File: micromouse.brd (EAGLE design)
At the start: 100 x 80 mm, 25 parts

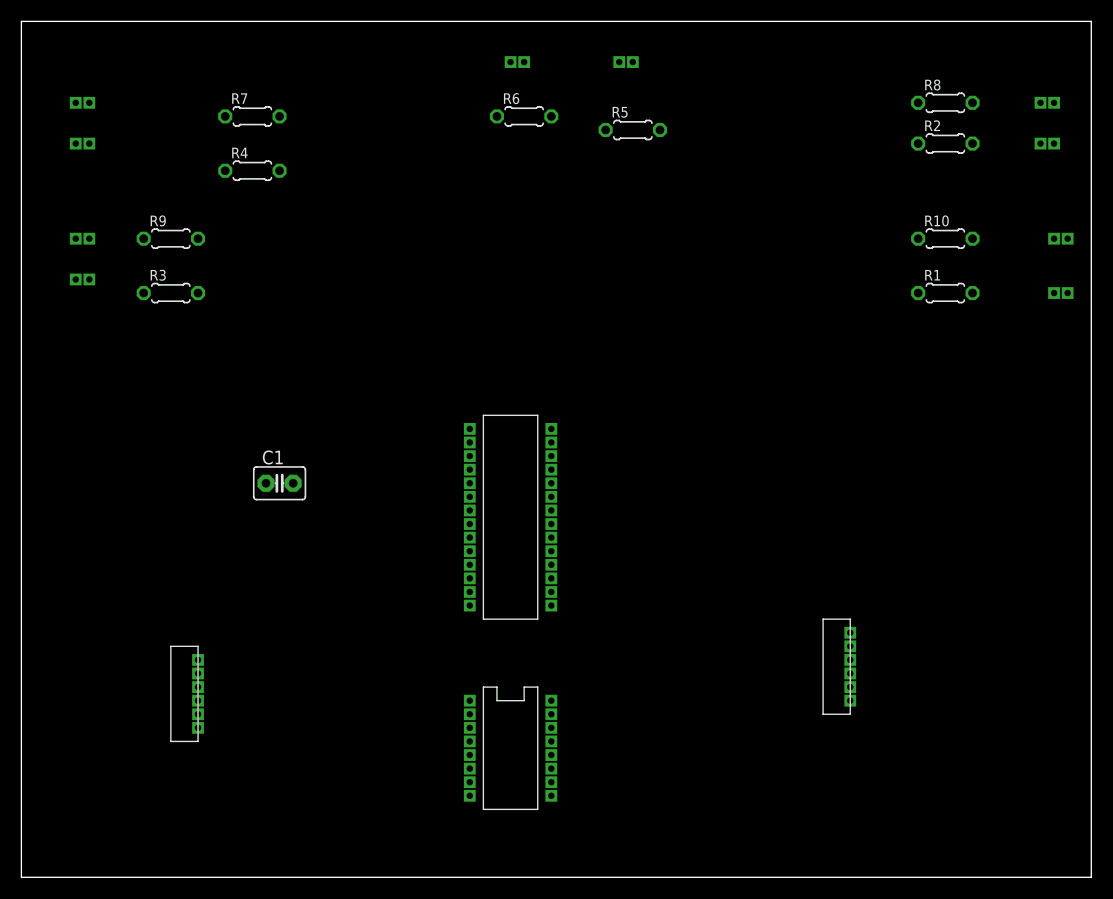
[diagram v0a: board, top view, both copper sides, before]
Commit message: Add files via upload
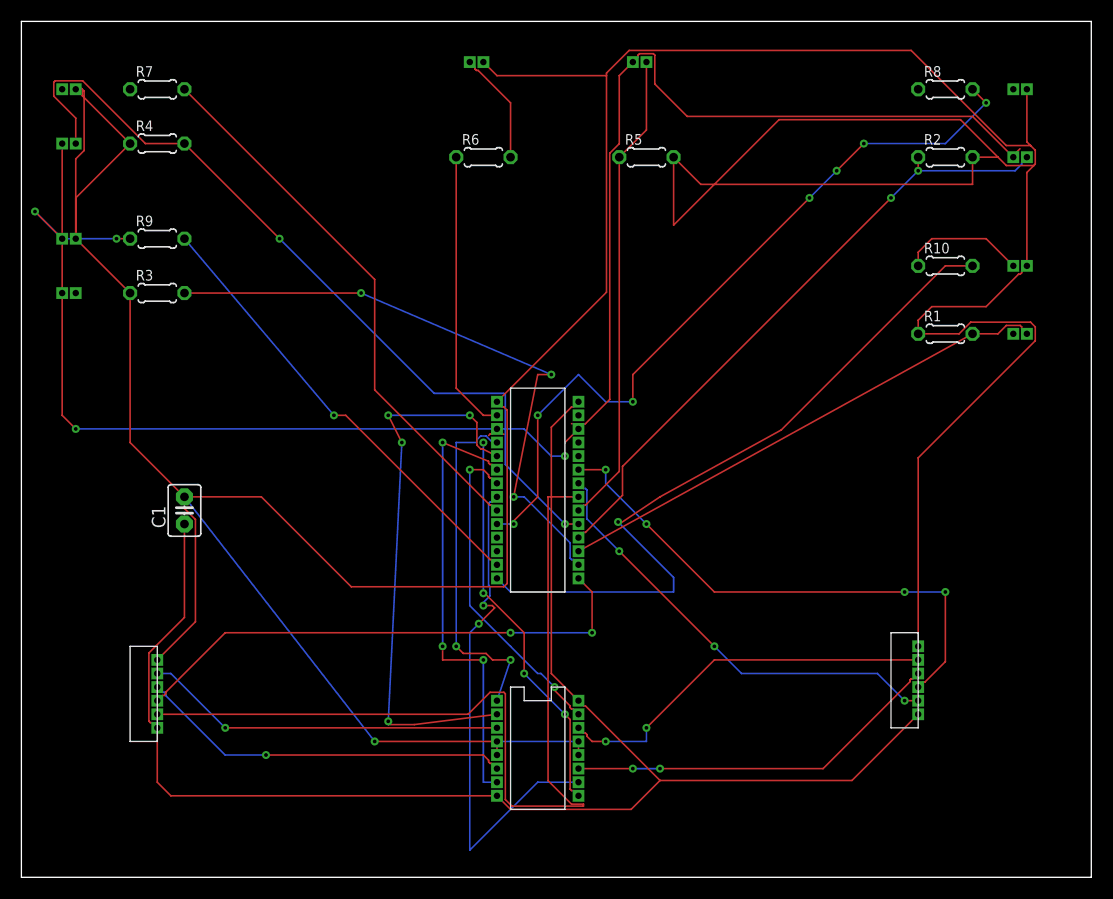
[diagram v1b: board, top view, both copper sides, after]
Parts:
- moved C1 9.25 mm to (15.2, 34.3), turned to 90 degrees
- moved R4 9.25 mm to (12.7, 68.6)
- moved R7 9.25 mm to (12.7, 73.7)
- moved U$14 6.48 mm to (85.1, 19.1)
- moved R6 5.39 mm to (43.2, 67.3)
- moved U$4 5.39 mm to (94.0, 50.8)
- moved U$12 4.58 mm to (94.0, 57.1)
- moved R1 3.81 mm to (86.4, 50.8)
- moved U$8 3.81 mm to (43.2, 76.2)
- moved U$13 3.81 mm to (14.0, 17.8)
- moved U$1 3.59 mm to (48.3, 36.8)
- moved R5 2.84 mm to (58.4, 67.3)
- moved U$10 2.84 mm to (94.0, 73.7)
- moved U$5 2.84 mm to (94.0, 67.3)
- moved R10 2.54 mm to (86.4, 57.1)
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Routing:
- net GND: track 0.00 -> 428.1 mm, vias 0 -> 1
- net N$36: track 0.00 -> 156.3 mm, vias 0 -> 2
- net N$30: track 0.00 -> 142.6 mm
- net N$29: track 0.00 -> 84.7 mm
- net N$21: track 0.00 -> 77.5 mm, vias 0 -> 2
- net N$14: track 0.00 -> 72.5 mm, vias 0 -> 7
- net N$18: track 0.00 -> 67.7 mm, vias 0 -> 1
- net N$20: track 0.00 -> 59.6 mm, vias 0 -> 2
- net N$24: track 0.00 -> 58.6 mm, vias 0 -> 4
- net N$2: track 0.00 -> 52.3 mm, vias 0 -> 4
- net N$12: track 0.00 -> 51.6 mm
- net N$28: track 0.00 -> 49.8 mm, vias 0 -> 4
- net N$27: track 0.00 -> 49.0 mm, vias 0 -> 2
- net N$7: track 0.00 -> 48.7 mm, vias 0 -> 2
- net N$19: track 0.00 -> 48.6 mm
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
